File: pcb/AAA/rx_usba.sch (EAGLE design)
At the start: 32 parts, among them Y1 CRYSTAL-26MHZSMD-3.2X2.5

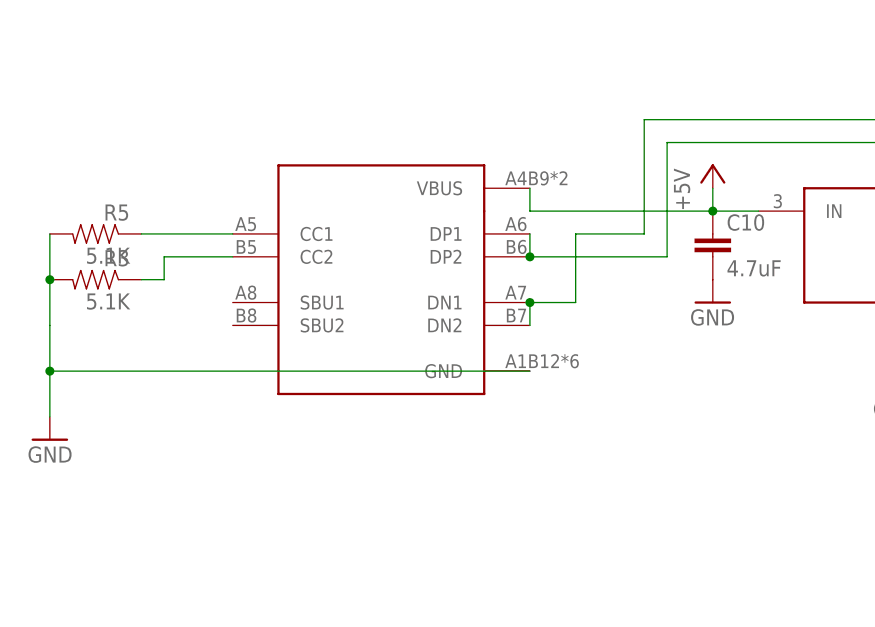
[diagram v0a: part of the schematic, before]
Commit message: txrx rev2 finished
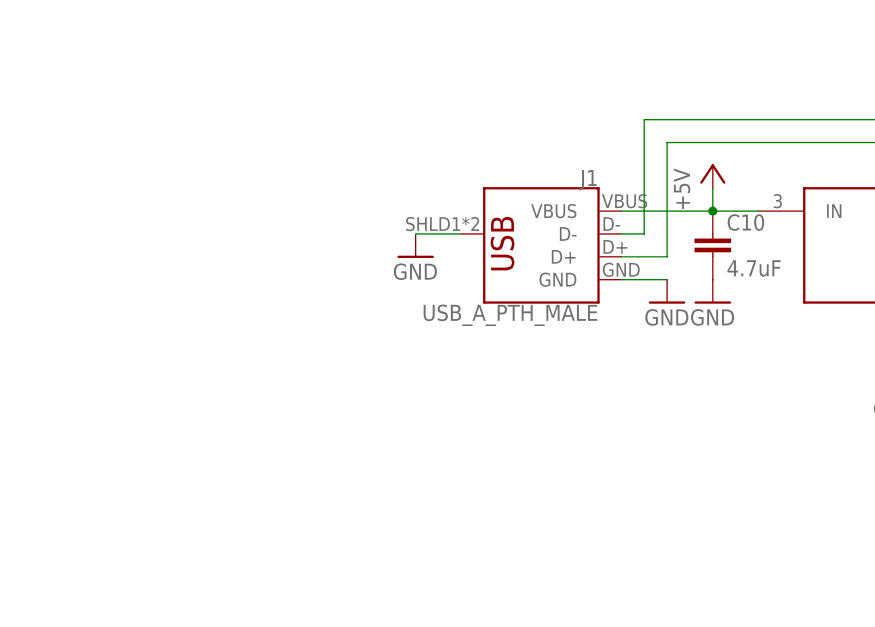
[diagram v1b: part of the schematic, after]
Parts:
- removed R3, R5: 5.1K, joyAnalog:RESISTOR0805-RES
- removed U$6: USBC_16P, my_usbc_16p:USBC_16P
- added J1: USB_A_PTH_MALE, rx20:USB_A_PTH_MALE
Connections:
- removed net N$25: R3.1, U$6.CC2
- removed net N$27: R5.1, U$6.CC1
- net +5V: now also J1.VBUS; no longer U$6.VBUS
- net GND: now also J1.GND, J1.SHIELD; no longer R3.2, R5.2, U$6.GND
- net N$12: now also J1.D-; no longer U$6.DN1, U$6.DN2
- net N$13: now also J1.D+; no longer U$6.DP1, U$6.DP2
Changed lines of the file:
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@@
 <parts>
 <part name="U$3" library="nRF24L01-Chip-v13" deviceset="NRF24L01" device="ALT1"/>
+<part name="J1" library="rx20" deviceset="USB_A" device="_PTH_MALE"/>
 <part name="GND14" library="supply1" library_urn="urn:adsk.eagle:library:371" deviceset="GND" device=""/>
 <part name="+3V10" library="supply1" library_urn="urn:adsk.eagle:library:371" deviceset="+3V3" device=""/>
@@
 <part name="GND11" library="clock" deviceset="GND" device=""/>
 <part name="U$4" library="3pos_slide_switch" deviceset="XC6206_DEV" device=""/>
+<part name="GND13" library="supply1" library_urn="urn:adsk.eagle:library:371" deviceset="GND" device=""/>
+<part name="GND15" library="supply1" library_urn="urn:adsk.eagle:library:371" deviceset="GND" device=""/>
 <part name="C10" library="clock" deviceset="CAP" device="0805" value="4.7uF"/>
 <part name="C11" library="clock" deviceset="CAP" device="0805" value="4.7uF"/>
@@
 <part name="U$5" library="adafruit_changed" deviceset="PINHD5" device=""/>
 <part name="+3V5" library="supply1" library_urn="urn:adsk.eagle:library:371" deviceset="+3V3" device=""/>
-<part name="U$6" library="my_usbc_16p" deviceset="USBC_16P" device=""/>
-<part name="GND21" library="supply1" deviceset="GND" device=""/>
-<part name="R3" library="joyAnalog" deviceset="RESISTOR" device="0805-RES" value="5.1K"/>
-<part name="R5" library="joyAnalog" deviceset="RESISTOR" device="0805-RES" value="5.1K"/>
 </parts>
 <sheets>
@@
 <instances>
 <instance part="U$3" gate="G$1" x="119.38" y="12.7"/>
+<instance part="J1" gate="G$1" x="-154.94" y="-10.16" rot="MR0"/>
 <instance part="GND14" gate="1" x="-22.86" y="38.1" rot="R180"/>
 <instance part="+3V10" gate="G$1" x="-73.66" y="-2.54"/>
@@
 <instance part="GND11" gate="1" x="152.4" y="-33.02"/>
 <instance part="U$4" gate="G$1" x="-116.84" y="-7.62"/>
+<instance part="GND13" gate="1" x="-142.24" y="-15.24"/>
+<instance part="GND15" gate="1" x="-170.18" y="-10.16"/>
 <instance part="C10" gate="G$1" x="-137.16" y="-10.16"/>
 <instance part="C11" gate="G$1" x="-99.06" y="-10.16"/>
@@
 <instance part="U$5" gate="G$1" x="81.28" y="-7.62"/>
 <instance part="+3V5" gate="G$1" x="-30.48" y="22.86"/>
-<instance part="U$6" gate="G$1" x="-172.72" y="-22.86" rot="MR0"/>
-<instance part="GND21" gate="1" x="-210.82" y="-30.48" rot="MR0"/>
-<instance part="R3" gate="G$1" x="-205.74" y="-12.7" rot="MR0"/>
-<instance part="R5" gate="G$1" x="-205.74" y="-7.62" rot="MR0"/>
 </instances>
 <busses>
@@
 </segment>
 <segment>
+<pinref part="GND15" gate="1" pin="GND"/>
+<pinref part="J1" gate="G$1" pin="SHIELD"/>
+<wire x1="-170.18" y1="-7.62" x2="-165.1" y2="-7.62" width="0.1524" layer="91"/>
+</segment>
+<segment>
+<pinref part="J1" gate="G$1" pin="GND"/>
+<pinref part="GND13" gate="1" pin="GND"/>
+<wire x1="-147.32" y1="-12.7" x2="-142.24" y2="-12.7" width="0.1524" layer="91"/>
+</segment>
+<segment>
 <pinref part="C10" gate="G$1" pin="2"/>
 <pinref part="GND16" gate="1" pin="GND"/>
@@
 <wire x1="71.12" y1="-10.16" x2="78.74" y2="-10.16" width="0.1524" layer="91"/>
 <pinref part="U$5" gate="G$1" pin="5"/>
-</segment>
-<segment>
-<pinref part="GND21" gate="1" pin="GND"/>
-<wire x1="-210.82" y1="-17.78" x2="-210.82" y2="-22.86" width="0.1524" layer="91"/>
-<pinref part="R3" gate="G$1" pin="2"/>
-<wire x1="-210.82" y1="-22.86" x2="-210.82" y2="-27.94" width="0.1524" layer="91"/>
-<wire x1="-210.82" y1="-12.7" x2="-210.82" y2="-17.78" width="0.1524" layer="91"/>
-<junction x="-210.82" y="-12.7"/>
-<pinref part="R5" gate="G$1" pin="2"/>
-<wire x1="-210.82" y1="-7.62" x2="-210.82" y2="-12.7" width="0.1524" layer="91"/>
-<pinref part="U$6" gate="G$1" pin="GND"/>
-<wire x1="-157.48" y1="-22.86" x2="-210.82" y2="-22.86" width="0.1524" layer="91"/>
-<junction x="-210.82" y="-22.86"/>
 </segment>
 </net>
@@
 <segment>
 <wire x1="-144.78" y1="5.08" x2="-144.78" y2="-7.62" width="0.1524" layer="91"/>
+<pinref part="J1" gate="G$1" pin="D-"/>
+<wire x1="-144.78" y1="-7.62" x2="-147.32" y2="-7.62" width="0.1524" layer="91"/>
 <pinref part="U$2" gate="G$1" pin="PA9/PA11"/>
 <wire x1="-144.78" y1="5.08" x2="50.8" y2="5.08" width="0.1524" layer="91"/>
-<wire x1="-144.78" y1="-7.62" x2="-152.4" y2="-7.62" width="0.1524" layer="91"/>
-<wire x1="-152.4" y1="-7.62" x2="-152.4" y2="-15.24" width="0.1524" layer="91"/>
-<pinref part="U$6" gate="G$1" pin="DN1"/>
-<pinref part="U$6" gate="G$1" pin="DN2"/>
-<wire x1="-157.48" y1="-15.24" x2="-157.48" y2="-17.78" width="0.1524" layer="91"/>
-<wire x1="-152.4" y1="-15.24" x2="-157.48" y2="-15.24" width="0.1524" layer="91"/>
-<junction x="-157.48" y="-15.24"/>
 </segment>
 </net>
@@
 <segment>
 <wire x1="-142.24" y1="2.54" x2="-142.24" y2="-10.16" width="0.1524" layer="91"/>
+<pinref part="J1" gate="G$1" pin="D+"/>
+<wire x1="-142.24" y1="-10.16" x2="-147.32" y2="-10.16" width="0.1524" layer="91"/>
 <pinref part="U$2" gate="G$1" pin="PA10/PA12"/>
 <wire x1="50.8" y1="2.54" x2="-142.24" y2="2.54" width="0.1524" layer="91"/>
-<pinref part="U$6" gate="G$1" pin="DP1"/>
-<pinref part="U$6" gate="G$1" pin="DP2"/>
-<wire x1="-157.48" y1="-7.62" x2="-157.48" y2="-10.16" width="0.1524" layer="91"/>
-<wire x1="-142.24" y1="-10.16" x2="-157.48" y2="-10.16" width="0.1524" layer="91"/>
-<junction x="-157.48" y="-10.16"/>
 </segment>
 </net>
@@
 <net name="+5V" class="0">
 <segment>
+<pinref part="J1" gate="G$1" pin="VBUS"/>
 <pinref part="U$4" gate="G$1" pin="IN"/>
+<wire x1="-147.32" y1="-5.08" x2="-137.16" y2="-5.08" width="0.1524" layer="91"/>
 <pinref part="C10" gate="G$1" pin="1"/>
 <wire x1="-137.16" y1="-5.08" x2="-132.08" y2="-5.08" width="0.1524" layer="91"/>
@@
 <pinref part="P+1" gate="1" pin="+5V"/>
 <wire x1="-137.16" y1="-2.54" x2="-137.16" y2="-5.08" width="0.1524" layer="91"/>
-<pinref part="U$6" gate="G$1" pin="VBUS"/>
-<wire x1="-137.16" y1="-5.08" x2="-157.48" y2="-5.08" width="0.1524" layer="91"/>
-<wire x1="-157.48" y1="-5.08" x2="-157.48" y2="-2.54" width="0.1524" layer="91"/>
 </segment>
 </net>
@@
 </segment>
 </net>
-<net name="N$25" class="0">
-<segment>
-<pinref part="R3" gate="G$1" pin="1"/>
-<wire x1="-198.12" y1="-12.7" x2="-200.66" y2="-12.7" width="0.1524" layer="91"/>
-<wire x1="-190.5" y1="-10.16" x2="-198.12" y2="-10.16" width="0.1524" layer="91"/>
-<wire x1="-198.12" y1="-10.16" x2="-198.12" y2="-12.7" width="0.1524" layer="91"/>
-<pinref part="U$6" gate="G$1" pin="CC2"/>
-</segment>
-</net>
-<net name="N$27" class="0">
-<segment>
-<pinref part="R5" gate="G$1" pin="1"/>
-<wire x1="-190.5" y1="-7.62" x2="-200.66" y2="-7.62" width="0.1524" layer="91"/>
-<pinref part="U$6" gate="G$1" pin="CC1"/>
-</segment>
-</net>
